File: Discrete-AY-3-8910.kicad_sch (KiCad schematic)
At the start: 1 part, among them J1 Conn_01x20

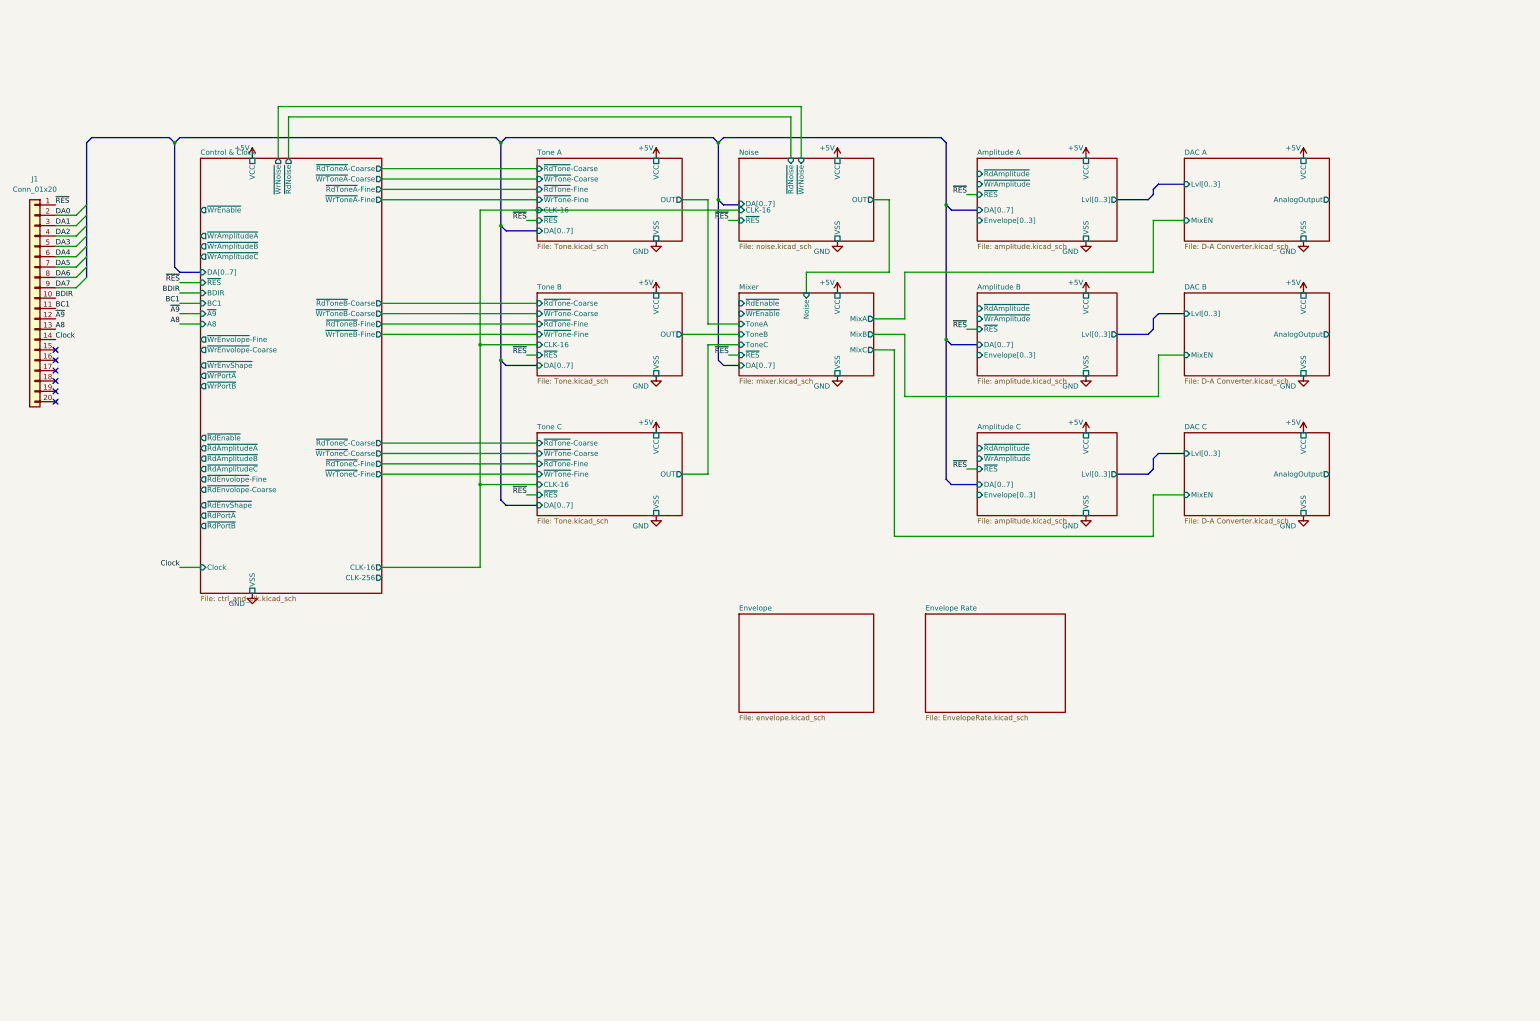
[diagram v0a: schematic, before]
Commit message: Fin de création de tous les schémas - envelope.kicad_sch - EnvelopeRate.kicad_sch
git-svn-id: file:///D%5C00%20-%20Dev%20&%20Calculs%5CRepoTortoiseSVN_PCB%5CRevivalChips/branches/Discrete-AY-3-8910@28 8d7748af-fe70-f644-8493-3f4b7ec62ef1
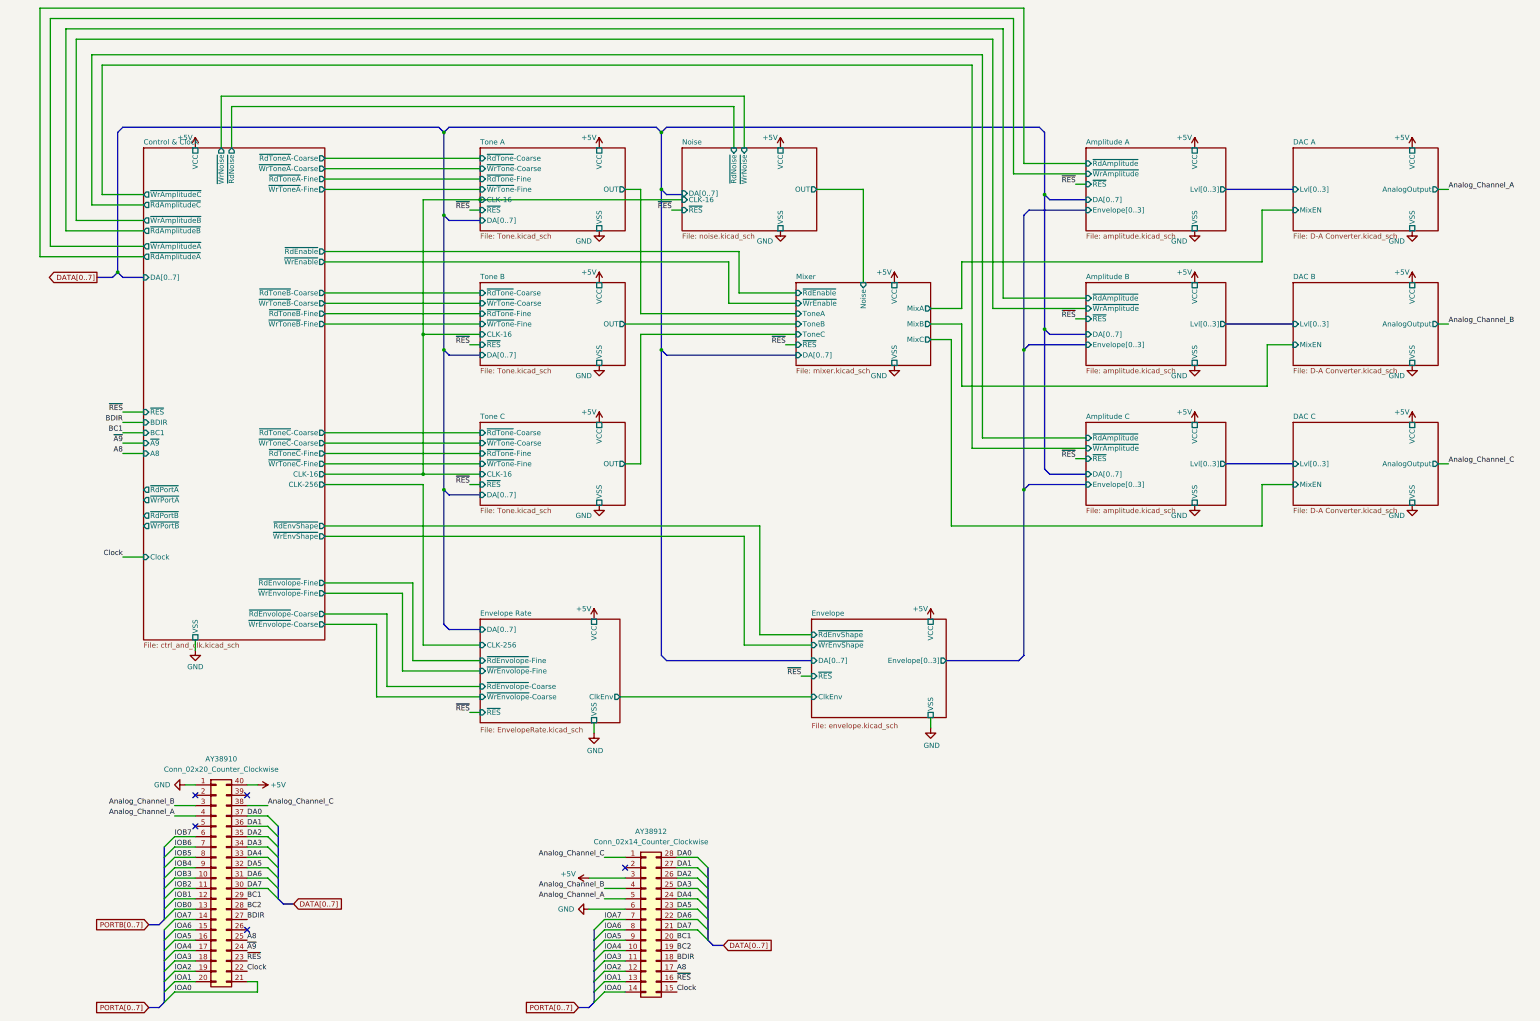
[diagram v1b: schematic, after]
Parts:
- removed J1: Conn_01x20, symbol Connector_Generic:Conn_01x20
- added AY38910: Conn_02x20_Counter_Clockwise, symbol Connector_Generic:Conn_02x20_Counter_Clockwise
- added AY38912: Conn_02x14_Counter_Clockwise, symbol Connector_Generic:Conn_02x14_Counter_Clockwise
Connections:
- net +5V: now also AY38910.40 (Pin_40), AY38912.3 (Pin_3)
- net A8: now also AY38910.25 (Pin_25), AY38912.17 (Pin_17)
- net BC1: now also AY38910.29 (Pin_29), AY38912.20 (Pin_20)
- net BDIR: now also AY38910.27 (Pin_27), AY38912.18 (Pin_18)
- net Clock: now also AY38910.22 (Pin_22), AY38912.15 (Pin_15)
- net DA0: now also AY38910.37 (Pin_37), AY38912.28 (Pin_28)
- net DA1: now also AY38910.36 (Pin_36), AY38912.27 (Pin_27)
- net DA2: now also AY38910.35 (Pin_35), AY38912.26 (Pin_26)
- net DA3: now also AY38910.34 (Pin_34), AY38912.25 (Pin_25)
- net DA4: now also AY38910.33 (Pin_33), AY38912.24 (Pin_24)
- net DA5: now also AY38910.32 (Pin_32), AY38912.23 (Pin_23)
- net DA6: now also AY38910.31 (Pin_31), AY38912.22 (Pin_22)
- net DA7: now also AY38910.30 (Pin_30), AY38912.21 (Pin_21)
- net GND: now also AY38910.1 (Pin_1), AY38912.6 (Pin_6)
- net ~{A9}: now also AY38910.24 (Pin_24)
- net ~{RES}: now also AY38910.23 (Pin_23), AY38912.16 (Pin_16)
- new net Analog_Channel_A: AY38910.4 (Pin_4), AY38912.5 (Pin_5)
- new net Analog_Channel_B: AY38910.3 (Pin_3), AY38912.4 (Pin_4)
- new net Analog_Channel_C: AY38910.38 (Pin_38), AY38912.1 (Pin_1)
- new net BC2: AY38910.28 (Pin_28), AY38912.19 (Pin_19)
- new net IOA0: AY38910.21 (Pin_21), AY38912.14 (Pin_14)
- new net IOA1: AY38910.20 (Pin_20), AY38912.13 (Pin_13)
- new net IOA2: AY38910.19 (Pin_19), AY38912.12 (Pin_12)
- new net IOA3: AY38910.18 (Pin_18), AY38912.11 (Pin_11)
- new net IOA4: AY38910.17 (Pin_17), AY38912.10 (Pin_10)
- new net IOA5: AY38910.16 (Pin_16), AY38912.9 (Pin_9)
- new net IOA6: AY38910.15 (Pin_15), AY38912.8 (Pin_8)
- new net IOA7: AY38910.14 (Pin_14), AY38912.7 (Pin_7)
- new net IOB0: AY38910.13 (Pin_13)
- new net IOB1: AY38910.12 (Pin_12)
- new net IOB2: AY38910.11 (Pin_11)
- new net IOB3: AY38910.10 (Pin_10)
- new net IOB4: AY38910.9 (Pin_9)
- new net IOB5: AY38910.8 (Pin_8)
- new net IOB6: AY38910.7 (Pin_7)
- new net IOB7: AY38910.6 (Pin_6)
- no-connect marks 6 -> 5
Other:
- sheet Envelope ports: added ClkEnv, DA[0..7], Envelope[0..3], VCC, VSS, ~{RES}, ~{RdEnvShape}, ~{WrEnvShape}; removed none
- sheet Envelope Rate ports: added CLK-256, ClkEnv, DA[0..7], VCC, VSS, ~{RES}, ~{RdEnvolope}-Coarse, ~{RdEnvolope}-Fine, ~{WrEnvolope}-Coarse, ~{WrEnvolope}-Fine; removed none
